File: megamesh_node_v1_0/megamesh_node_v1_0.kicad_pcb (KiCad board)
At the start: 2 copper layers, 85.5 x 60.5 mm, 4 parts, among them J1 Conn_Coaxial, U1 ESP32-S3-WROOM-1, U2 LoRa126XF30, U3 BQ25798

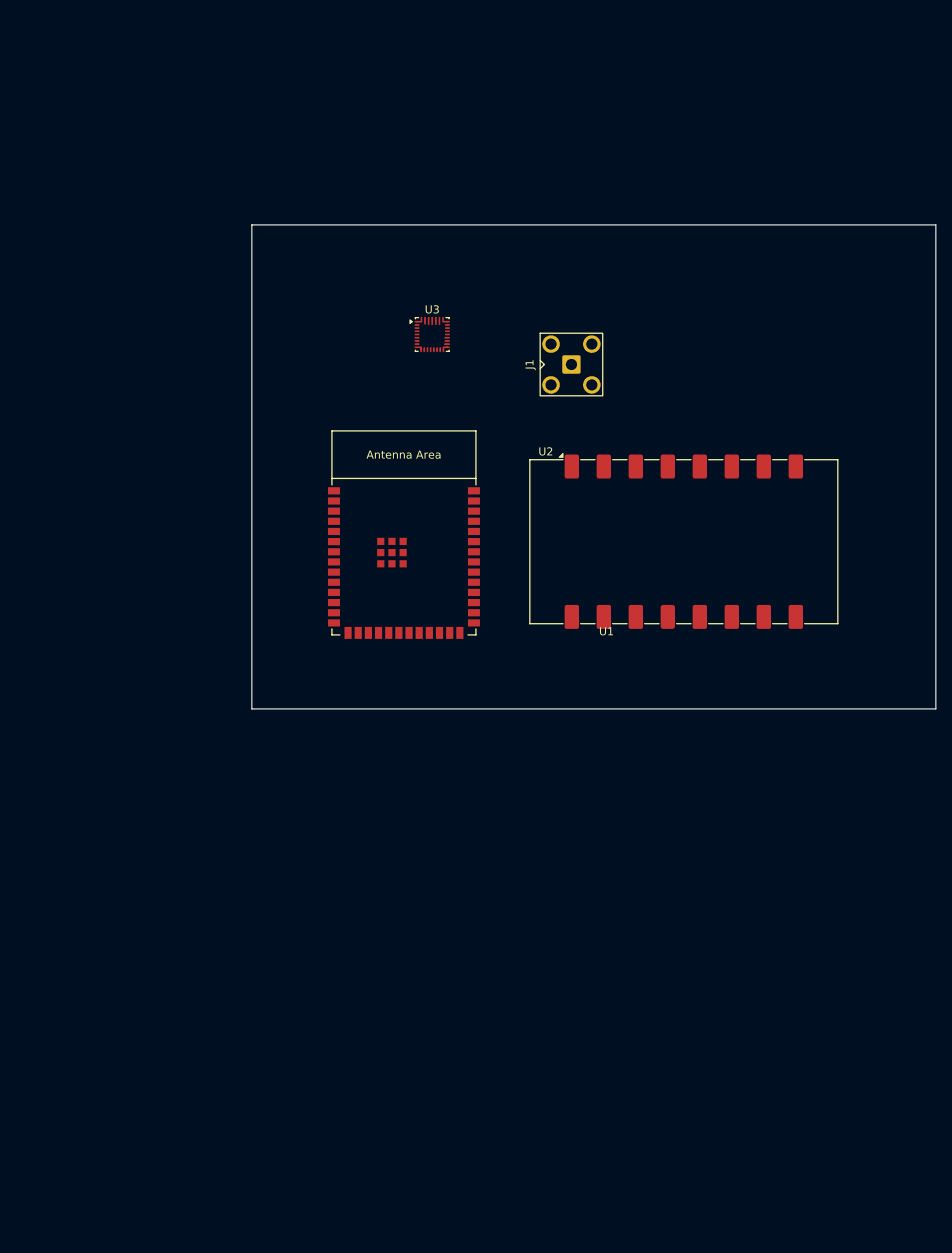
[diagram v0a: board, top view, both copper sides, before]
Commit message: Entwicklung Schaltplan und Platine
Es geht voran
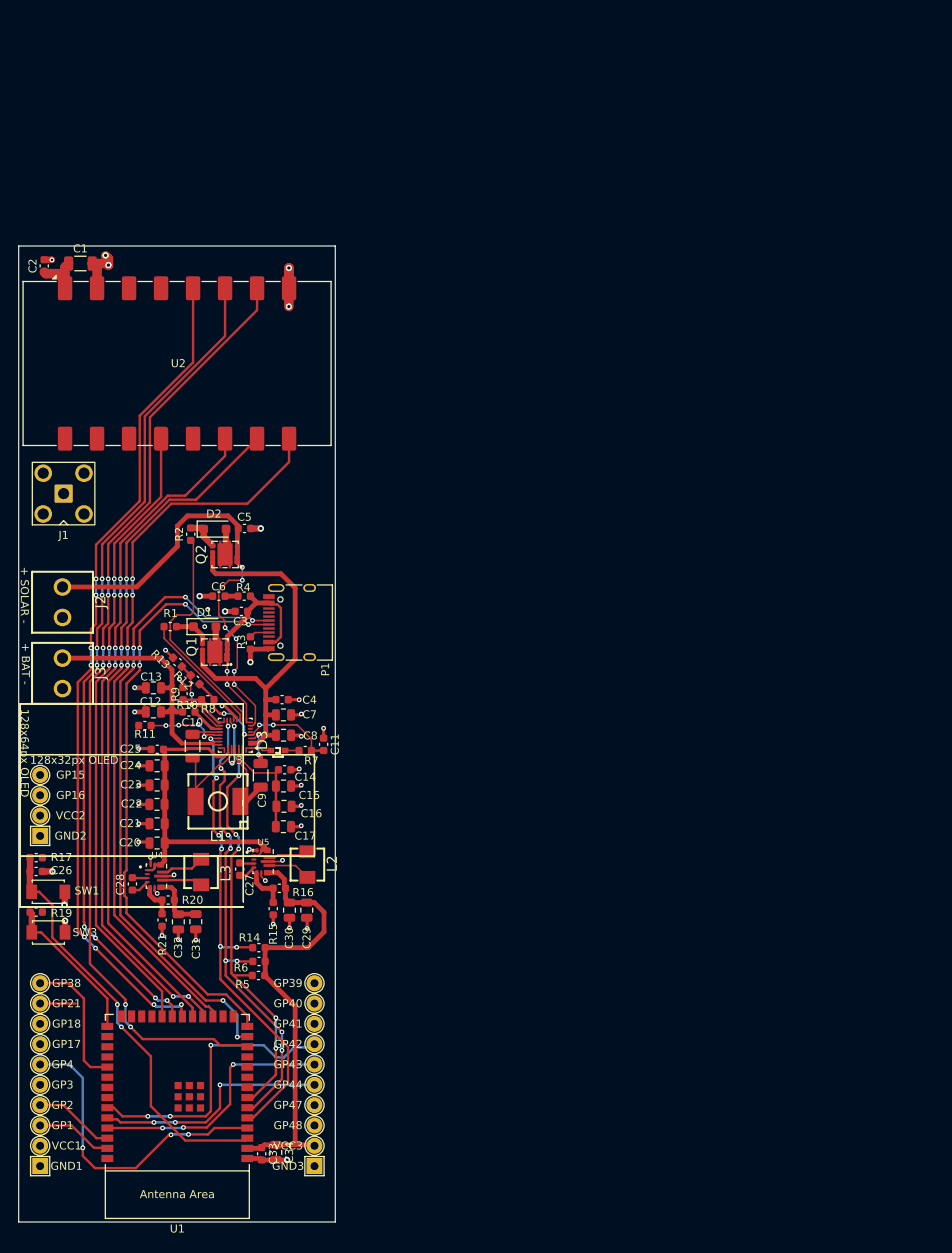
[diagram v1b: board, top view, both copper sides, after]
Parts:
- added C1: 47 uF, Capacitor_SMD:C_1206_3216Metric, F.Cu at (71.1, 71.3)
- added C10: 47 uF, Capacitor_SMD:C_1206_3216Metric, F.Cu at (85.1, 131.7)
- added C11: 47 nF, Capacitor_SMD:C_0603_1608Metric, F.Cu at (101.5, 131.4)
- added C12: 10 uF, Capacitor_SMD:C_0805_2012Metric, F.Cu at (80.2, 127.4)
- added C13: 10 uF, Capacitor_SMD:C_0805_2012Metric, F.Cu at (80.2, 124.4)
- added C14: 0.1 uF, Capacitor_SMD:C_0603_1608Metric, F.Cu at (96.6, 134.6)
- added C15: 10 uF, Capacitor_SMD:C_0805_2012Metric, F.Cu at (96.5, 136.6)
- added C16: 10 uF, Capacitor_SMD:C_0805_2012Metric, F.Cu at (96.5, 139.2)
- added C17: 10 uF, Capacitor_SMD:C_0805_2012Metric, F.Cu at (96.4, 141.7)
- added C2: 100 nF, Capacitor_SMD:C_0603_1608Metric, F.Cu at (66.5, 71.6)
- added C20: 10 uF, Capacitor_SMD:C_0805_2012Metric, F.Cu at (80.7, 143.8)
- added C21: 10 uF, Capacitor_SMD:C_0805_2012Metric, F.Cu at (80.7, 141.4)
- added C22: 10 uF, Capacitor_SMD:C_0805_2012Metric, F.Cu at (80.6, 138.9)
- added C23: 10 uF, Capacitor_SMD:C_0805_2012Metric, F.Cu at (80.7, 136.5)
- added C24: 10 uF, Capacitor_SMD:C_0805_2012Metric, F.Cu at (80.7, 134.1)
- added C25: 0.1 uF, Capacitor_SMD:C_0603_1608Metric, F.Cu at (80.7, 132.1)
- added C26: 100 nF, Capacitor_SMD:C_0603_1608Metric, F.Cu at (65.5, 147.3)
- added C27: 1 uF, Capacitor_SMD:C_0603_1608Metric, F.Cu at (91.0, 147.0)
- added C28: 1 uF, Capacitor_SMD:C_0603_1608Metric, F.Cu at (77.6, 148.9)
- added C29: 22 uF, Capacitor_SMD:C_0805_2012Metric, F.Cu at (99.4, 152.2)
- added C3: 0.1uF, Capacitor_SMD:C_0603_1608Metric, F.Cu at (91.2, 114.8)
- added C30: 22 uF, Capacitor_SMD:C_0805_2012Metric, F.Cu at (97.2, 152.2)
- added C31: 22 uF, Capacitor_SMD:C_0805_2012Metric, F.Cu at (85.5, 153.6)
- added C32: 22 uF, Capacitor_SMD:C_0805_2012Metric, F.Cu at (83.3, 153.6)
- added C33: 100 nF, Capacitor_SMD:C_0603_1608Metric, F.Cu at (93.7, 182.6)
- added C34: 10 uF, Capacitor_SMD:C_0805_2012Metric, F.Cu at (95.5, 182.4)
- added C4: 0.1 uF, Capacitor_SMD:C_0603_1608Metric, F.Cu at (96.3, 125.8)
- added C5: 0.1uF, Capacitor_SMD:C_0603_1608Metric, F.Cu at (91.6, 104.4)
- added C6: 2.2 uF, Capacitor_SMD:C_0603_1608Metric, F.Cu at (88.4, 112.9)
- added C7: 10 uF, Capacitor_SMD:C_0805_2012Metric, F.Cu at (96.5, 127.7)
- added C8: 10 uF, Capacitor_SMD:C_0805_2012Metric, F.Cu at (96.5, 130.3)
- added C9: 47 uF, Capacitor_SMD:C_1206_3216Metric, F.Cu at (93.6, 135.3)
- added D1: BZT52BC12, Diode_SMD:D_SOD-123F, F.Cu at (86.6, 116.7)
- added D2: BZT52BC12, Diode_SMD:D_SOD-123F, F.Cu at (87.9, 104.5)
- added D3: LED, myRF:LED-SMD_L1.7-W0.6-R-RD, F.Cu at (95.8, 132.2)
- added GND1: GND, TestPoint:TestPoint_THTPad_2.0x2.0mm_Drill1.0mm, F.Cu at (66.0, 184.2)
- added GND2: GND, TestPoint:TestPoint_THTPad_2.0x2.0mm_Drill1.0mm, F.Cu at (66.0, 142.9)
- added GND3: GND, TestPoint:TestPoint_THTPad_2.0x2.0mm_Drill1.0mm, F.Cu at (100.3, 184.2)
- added GP1: GPIO1, TestPoint:TestPoint_THTPad_D2.0mm_Drill1.0mm, F.Cu at (66.0, 179.1)
- added GP15: I2C SDA, TestPoint:TestPoint_THTPad_D2.0mm_Drill1.0mm, F.Cu at (66.0, 135.3)
- added GP16: I2C SCL, TestPoint:TestPoint_THTPad_D2.0mm_Drill1.0mm, F.Cu at (66.0, 137.8)
- added GP17: GPIO17, TestPoint:TestPoint_THTPad_D2.0mm_Drill1.0mm, F.Cu at (66.0, 168.9)
- added GP18: GPIO18, TestPoint:TestPoint_THTPad_D2.0mm_Drill1.0mm, F.Cu at (66.0, 166.4)
- added GP2: GPIO2, TestPoint:TestPoint_THTPad_D2.0mm_Drill1.0mm, F.Cu at (66.0, 176.5)
- added GP21: GPIO21, TestPoint:TestPoint_THTPad_D2.0mm_Drill1.0mm, F.Cu at (66.0, 163.8)
- added GP3: GPIO3, TestPoint:TestPoint_THTPad_D2.0mm_Drill1.0mm, F.Cu at (66.0, 174.0)
- added GP38: GPIO38, TestPoint:TestPoint_THTPad_D2.0mm_Drill1.0mm, F.Cu at (66.0, 161.3)
- added GP39: GPIO39, TestPoint:TestPoint_THTPad_D2.0mm_Drill1.0mm, F.Cu at (100.3, 161.3)
- added GP4: GPIO4, TestPoint:TestPoint_THTPad_D2.0mm_Drill1.0mm, F.Cu at (66.0, 171.4)
- added GP40: GPIO40, TestPoint:TestPoint_THTPad_D2.0mm_Drill1.0mm, F.Cu at (100.3, 163.8)
- added GP41: GPIO41, TestPoint:TestPoint_THTPad_D2.0mm_Drill1.0mm, F.Cu at (100.3, 166.4)
- added GP42: GPIO42, TestPoint:TestPoint_THTPad_D2.0mm_Drill1.0mm, F.Cu at (100.3, 168.9)
- added GP43: TX0, TestPoint:TestPoint_THTPad_D2.0mm_Drill1.0mm, F.Cu at (100.3, 171.4)
- added GP44: RX0, TestPoint:TestPoint_THTPad_D2.0mm_Drill1.0mm, F.Cu at (100.3, 174.0)
- added GP47: GPIO47, TestPoint:TestPoint_THTPad_D2.0mm_Drill1.0mm, F.Cu at (100.3, 176.5)
- added GP48: GPIO48, TestPoint:TestPoint_THTPad_D2.0mm_Drill1.0mm, F.Cu at (100.3, 179.1)
- added J2: Screw_Terminal_01x02, myRF:CONN-TH_2P-P3.81_KF124-3.81-2P, F.Cu at (68.8, 113.7)
- added J3: Screw_Terminal_01x02, myRF:CONN-TH_2P-P3.81_KF124-3.81-2P, F.Cu at (68.8, 122.6)
- added L1: 1.0 uH, myRF:IND-SMD_L7.1-W6.5-P5.60, F.Cu at (88.3, 138.6)
- added L2: 1.5 uH, myRF:IND-SMD_L4.2-W4.0_SPM4030T, F.Cu at (99.4, 146.5)
- added L3: 1.5 uH, myRF:IND-SMD_L4.2-W4.0_SPM4030T, F.Cu at (86.2, 147.4)
- added P1: USB_C_Plug_USB2.0, Connector_USB:USB_C_Receptacle_HRO_TYPE-C-31-M-12, F.Cu at (98.7, 116.2)
- added Q1: CSD87312Q3E, myRF:SON 3.3x3.3mm, F.Cu at (87.9, 119.9)
- added Q2: CSD87312Q3E, myRF:SON 3.3x3.3mm, F.Cu at (89.2, 107.7)
- added R1: 294 Ohm, Capacitor_SMD:C_0603_1608Metric, F.Cu at (82.3, 116.7)
- added R10: 100 Ohm, Capacitor_SMD:C_0603_1608Metric, F.Cu at (84.6, 127.4)
- added R11: 6.04 kOhm, Capacitor_SMD:C_0603_1608Metric, F.Cu at (79.1, 129.1)
- added R12: 127 kOhm, Capacitor_SMD:C_0603_1608Metric, F.Cu at (85.4, 123.4)
- added R13: 127 kOhm, Capacitor_SMD:C_0603_1608Metric, F.Cu at (83.2, 121.2)
- added R14: 4.7 kOhm, Capacitor_SMD:C_0603_1608Metric, F.Cu at (93.4, 156.8)
- added R15: 200 kOhm, Capacitor_SMD:C_0603_1608Metric, F.Cu at (95.2, 152.0)
- added R16: 624 kOhm, Capacitor_SMD:C_0603_1608Metric, F.Cu at (95.9, 149.4)
- added R17: 10 kOhm, Capacitor_SMD:C_0603_1608Metric, F.Cu at (65.5, 145.6)
- added R19: 10 kOhm, Capacitor_SMD:C_0603_1608Metric, F.Cu at (65.5, 152.4)
- added R2: 294 Ohm, Capacitor_SMD:C_0603_1608Metric, F.Cu at (84.9, 105.2)
- added R20: 649 kOhm, Capacitor_SMD:C_0603_1608Metric, F.Cu at (82.0, 150.9)
- added R21: 100 kOhm, Capacitor_SMD:C_0603_1608Metric, F.Cu at (81.3, 153.4)
- added R3: 5.1 kOhm, Capacitor_SMD:C_0603_1608Metric, F.Cu at (92.3, 118.8)
- added R4: 2 Ohm, Capacitor_SMD:C_0603_1608Metric, F.Cu at (91.5, 112.9)
- added R5: 4.7 kOhm, Capacitor_SMD:C_0603_1608Metric, F.Cu at (93.3, 160.3)
- added R6: 4.7 kOhm, Capacitor_SMD:C_0603_1608Metric, F.Cu at (93.4, 158.6)
- added R7: 2.2 kOhm, Capacitor_SMD:C_0603_1608Metric, F.Cu at (99.2, 132.2)
- added R8: 10 kOhm, Capacitor_SMD:C_0603_1608Metric, F.Cu at (87.0, 125.9)
- added R9: 10 kOhm, Capacitor_SMD:C_0603_1608Metric, F.Cu at (83.9, 125.1)
- added SW1: SW_Push, myRF:SW_TS-1088-AR02016, F.Cu at (67.1, 149.9)
- added SW3: SW_Push, myRF:SW_TS-1088-AR02016, F.Cu at (67.1, 154.9)
- added U4: TPS63070RNMR, TPS63070RNMR:VREG_TPS63070RNMR, F.Cu at (80.6, 147.9)
- added U5: TPS63070RNMR, TPS63070RNMR:VREG_TPS63070RNMR, F.Cu at (93.9, 146.1)
- added VCC1: 3v3, TestPoint:TestPoint_THTPad_D2.0mm_Drill1.0mm, F.Cu at (66.0, 181.6)
- added VCC2: 3v3, TestPoint:TestPoint_THTPad_D2.0mm_Drill1.0mm, F.Cu at (66.0, 140.3)
- added VCC3: 3v3, TestPoint:TestPoint_THTPad_D2.0mm_Drill1.0mm, F.Cu at (100.3, 181.6)
- moved U1 72.7 mm to (83.2, 174.9), turned to 180 degrees
- moved U2 67.1 mm to (83.2, 83.8)
- moved J1 65.5 mm to (69.0, 100.1), turned to 90 degrees
- moved U3 55.8 mm to (90.4, 130.3), turned to 180 degrees
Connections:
- net Net-(U3-VBUS-Pad2) renamed D2
- U1 pad 10: unconnected-(U1-GPIO17/U1TXD/ADC2_CH6-Pad10) -> Net-(U1-GPIO17/U1TXD/ADC2_CH6)
- U1 pad 11: unconnected-(U1-GPIO18/U1RXD/ADC2_CH7/CLK_OUT3-Pad11) -> Net-(U1-GPIO18/U1RXD/ADC2_CH7/CLK_OUT3)
- U1 pad 12: unconnected-(U1-GPIO8/TOUCH8/ADC1_CH7/SUBSPICS1-Pad12) -> NSS
- U1 pad 13: unconnected-(U1-GPIO19/U1RTS/ADC2_CH8/CLK_OUT2/USB_D--Pad13) -> D-
- U1 pad 14: unconnected-(U1-GPIO20/U1CTS/ADC2_CH9/CLK_OUT1/USB_D+-Pad14) -> D+
- U1 pad 15: unconnected-(U1-GPIO3/TOUCH3/ADC1_CH2-Pad15) -> Net-(U1-GPIO3/TOUCH3/ADC1_CH2)
- U1 pad 17: unconnected-(U1-GPIO9/TOUCH9/ADC1_CH8/FSPIHD/SUBSPIHD-Pad17) -> SCK
- U1 pad 18: unconnected-(U1-GPIO10/TOUCH10/ADC1_CH9/FSPICS0/FSPIIO4/SUBSPICS0-Pad18) -> MOSI
- U1 pad 19: unconnected-(U1-GPIO11/TOUCH11/ADC2_CH0/FSPID/FSPIIO5/SUBSPID-Pad19) -> MISO
- U1 pad 2: unconnected-(U1-3V3-Pad2) -> +3V3
- U1 pad 20: unconnected-(U1-GPIO12/TOUCH12/ADC2_CH1/FSPICLK/FSPIIO6/SUBSPICLK-Pad20) -> NRESET
- U1 pad 21: unconnected-(U1-GPIO13/TOUCH13/ADC2_CH2/FSPIQ/FSPIIO7/SUBSPIQ-Pad21) -> BUSY
- U1 pad 22: unconnected-(U1-GPIO14/TOUCH14/ADC2_CH3/FSPIWP/FSPIDQS/SUBSPIWP-Pad22) -> DIO0
- U1 pad 23: unconnected-(U1-GPIO21-Pad23) -> Net-(U1-GPIO21)
- U1 pad 24: unconnected-(U1-GPIO47/SPICLK_P/SUBSPICLK_P_DIFF-Pad24) -> Net-(U1-GPIO47/SPICLK_P/SUBSPICLK_P_DIFF)
- U1 pad 25: unconnected-(U1-GPIO48/SPICLK_N/SUBSPICLK_N_DIFF-Pad25) -> Net-(U1-GPIO48/SPICLK_N/SUBSPICLK_N_DIFF)
- U1 pad 27: unconnected-(U1-GPIO0/BOOT-Pad27) -> BOOT_SW
- U1 pad 3: unconnected-(U1-EN-Pad3) -> EN_SW
- U1 pad 31: unconnected-(U1-GPIO38/FSPIWP/SUBSPIWP-Pad31) -> Net-(U1-GPIO38/FSPIWP/SUBSPIWP)
- U1 pad 32: unconnected-(U1-MTCK/GPIO39/CLK_OUT3/SUBSPICS1-Pad32) -> Net-(U1-MTCK/GPIO39/CLK_OUT3/SUBSPICS1)
- U1 pad 33: unconnected-(U1-MTDO/GPIO40/CLK_OUT2-Pad33) -> Net-(U1-MTDO/GPIO40/CLK_OUT2)
- U1 pad 34: unconnected-(U1-MTDI/GPIO41/CLK_OUT1-Pad34) -> Net-(U1-MTDI/GPIO41/CLK_OUT1)
- U1 pad 35: unconnected-(U1-MTMS/GPIO42-Pad35) -> Net-(U1-MTMS/GPIO42)
- U1 pad 36: unconnected-(U1-U0RXD/GPIO44/CLK_OUT2-Pad36) -> Net-(U1-U0RXD/GPIO44/CLK_OUT2)
- U1 pad 37: unconnected-(U1-U0TXD/GPIO43/CLK_OUT1-Pad37) -> Net-(U1-U0TXD/GPIO43/CLK_OUT1)
- U1 pad 38: unconnected-(U1-GPIO2/TOUCH2/ADC1_CH1-Pad38) -> Net-(U1-GPIO2/TOUCH2/ADC1_CH1)
- U1 pad 39: unconnected-(U1-GPIO1/TOUCH1/ADC1_CH0-Pad39) -> Net-(U1-GPIO1/TOUCH1/ADC1_CH0)
- U1 pad 4: unconnected-(U1-GPIO4/TOUCH4/ADC1_CH3-Pad4) -> Net-(U1-GPIO4/TOUCH4/ADC1_CH3)
- U1 pad 5: unconnected-(U1-GPIO5/TOUCH5/ADC1_CH4-Pad5) -> !INT
- U1 pad 6: unconnected-(U1-GPIO6/TOUCH6/ADC1_CH5-Pad6) -> SDA
- U1 pad 7: unconnected-(U1-GPIO7/TOUCH7/ADC1_CH6-Pad7) -> SCL
- U1 pad 8: unconnected-(U1-GPIO15/U0RTS/ADC2_CH4/XTAL_32K_P-Pad8) -> Net-(U1-GPIO15/U0RTS/ADC2_CH4/XTAL_32K_P)
- U1 pad 9: unconnected-(U1-GPIO16/U0CTS/ADC2_CH5/XTAL_32K_N-Pad9) -> Net-(U1-GPIO16/U0CTS/ADC2_CH5/XTAL_32K_N)
- U2 pad 1: +5V -> +6V
- U2 pad 10: unconnected-(U2-MISO-Pad10) -> MISO
- U2 pad 11: unconnected-(U2-MOSI-Pad11) -> MOSI
- U2 pad 13: unconnected-(U2-DIO1-Pad13) -> DIO0
- U2 pad 5: unconnected-(U2-NRESET-Pad5) -> NRESET
- U2 pad 6: unconnected-(U2-BUSY-Pad6) -> BUSY
- U2 pad 7: unconnected-(U2-NSS-Pad7) -> NSS
- U2 pad 8: unconnected-(U2-GND-Pad8) -> GND
- U2 pad 9: unconnected-(U2-SCK-Pad9) -> SCK
- U3 pad 1: unconnected-(U3-STAT-Pad1) -> Net-(D3-K)
- U3 pad 10: unconnected-(U3-ACDRV2-Pad10) -> Gate_ACDRV2
- U3 pad 11: unconnected-(U3-ACDRV1-Pad11) -> Gate_ACDRV1
- U3 pad 12: unconnected-(U3-~{QON}-Pad12) -> GND
- U3 pad 13: unconnected-(U3-~{CE}-Pad13) -> GND
- U3 pad 14: unconnected-(U3-SCL-Pad14) -> SCL
- U3 pad 15: unconnected-(U3-SDA-Pad15) -> SDA
- U3 pad 16: unconnected-(U3-TS-Pad16) -> Net-(U3-TS)
- U3 pad 17: unconnected-(U3-ILIM_HIZ-Pad17) -> Net-(U3-ILIM_HIZ)
- U3 pad 18: unconnected-(U3-BATP-Pad18) -> Net-(U3-BATP)
- U3 pad 19: unconnected-(U3-BTST2-Pad19) -> Net-(U3-BTST2)
- U3 pad 20: unconnected-(U3-PROG-Pad20) -> Net-(U3-PROG)
- U3 pad 21: unconnected-(U3-~{INT}-Pad21) -> !INT
- U3 pad 25: unconnected-(U3-SYS-Pad25) -> SYS
- U3 pad 26: unconnected-(U3-SW2-Pad26) -> Net-(U3-SW2)
- U3 pad 28: unconnected-(U3-SW1-Pad28) -> Net-(U3-SW1)
- U3 pad 29: unconnected-(U3-PMID-Pad29) -> Net-(U3-PMID)
- U3 pad 4: unconnected-(U3-BTST1-Pad4) -> Net-(U3-BTST1)
- U3 pad 5: unconnected-(U3-REGN-Pad5) -> REGN
- U3 pad 8: unconnected-(U3-VAC2-Pad8) -> D1_VAC2
- U3 pad 9: unconnected-(U3-VAC1-Pad9) -> D1_VAC1
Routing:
- net NSS: track 0.00 -> 118.7 mm, vias 0 -> 6
- net NRESET: track 0.00 -> 105.2 mm, vias 0 -> 8
- net BUSY: track 0.00 -> 103.5 mm, vias 0 -> 8
- net SCK: track 0.00 -> 92.2 mm, vias 0 -> 4
- net MOSI: track 0.00 -> 86.3 mm, vias 0 -> 6
- net MISO: track 0.00 -> 86.2 mm, vias 0 -> 4
- net GND: track 0.00 -> 84.4 mm, vias 0 -> 47
- net D-: track 0.00 -> 80.1 mm, vias 0 -> 6
- net DIO0: track 0.00 -> 79.0 mm, vias 0 -> 4
- net D+: track 0.00 -> 76.5 mm, vias 0 -> 4
- net !INT: track 0.00 -> 59.8 mm, vias 0 -> 6
- net SDA: track 0.00 -> 58.9 mm, vias 0 -> 8
- net D1_VAC2: track 0.00 -> 57.4 mm, vias 0 -> 6
- net +3V3: track 0.00 -> 56.0 mm
- net SCL: track 0.00 -> 55.8 mm, vias 0 -> 6
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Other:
- board size 85.5 x 60.5 mm -> 39.6 x 122 mm
- board text added: "+ BAT -"
- board text added: "+ SOLAR -"
- board text added: "128x32px OLED"
- board text added: "128x64px OLED"

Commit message: Fertigstellung
I guess
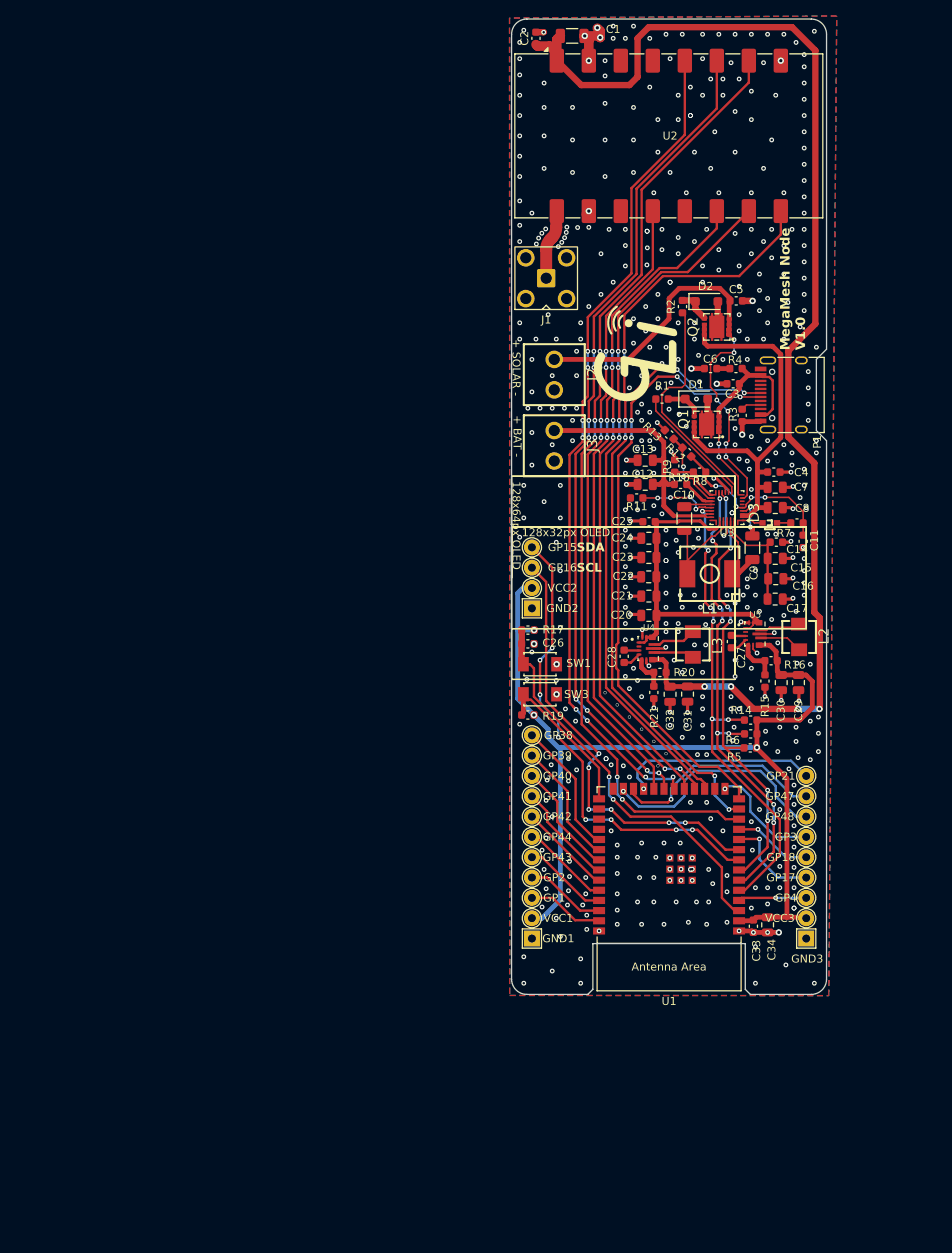
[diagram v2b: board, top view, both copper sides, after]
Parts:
- added G***: LOGO, LOGO, F.Cu at (140.5, 82.5)
- moved GP3 100.6 mm to (161.8, 143.0)
- moved GP21 99.9 mm to (161.8, 135.4)
- moved GP17 98.0 mm to (161.8, 148.1)
- moved GP18 98.0 mm to (161.8, 145.5)
- moved GP4 98.0 mm to (161.8, 150.6)
- moved GP47 72.6 mm to (161.8, 137.9)
- moved GP48 72.6 mm to (161.8, 140.5)
- moved GP38 68.8 mm to (127.5, 130.3)
- moved SW3 68.3 mm to (128.5, 125.2)
- moved C15 67.7 mm to (157.9, 108.2)
- moved C3 67.7 mm to (152.7, 86.4)
- moved R5 67.7 mm to (154.8, 131.9)
- moved U5 67.7 mm to (155.4, 117.6)
- moved C28 67.7 mm to (139.0, 120.4)
- moved C30 67.7 mm to (158.7, 123.7)
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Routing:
- net +6V: track 14.5 -> 158.2 mm, vias 0 -> 4
- net +3V3: track 56.0 -> 129.5 mm, vias 0 -> 3
- net Net-(U1-GPIO15/U0RTS/ADC2_CH4/XTAL_32K_P): track 0.00 -> 59.1 mm, vias 0 -> 8
- net Net-(U1-GPIO16/U0CTS/ADC2_CH5/XTAL_32K_N): track 0.00 -> 55.1 mm, vias 0 -> 6
- net Net-(U1-GPIO4/TOUCH4/ADC1_CH3): track 39.1 -> 8.53 mm, vias 3 -> 1
- net Net-(U1-GPIO48/SPICLK_N/SUBSPICLK_N_DIFF): track 0.00 -> 30.1 mm, vias 0 -> 1
- net Net-(U1-GPIO47/SPICLK_P/SUBSPICLK_P_DIFF): track 0.00 -> 27.0 mm, vias 0 -> 1
- net Net-(U1-MTMS/GPIO42): track 36.3 -> 11.7 mm, vias 3 -> 0
- net Net-(U1-U0TXD/GPIO43/CLK_OUT1): track 32.0 -> 10.6 mm, vias 3 -> 0
- net Net-(U1-GPIO21): track 4.44 -> 25.0 mm, vias 0 -> 1
- net Net-(U1-U0RXD/GPIO44/CLK_OUT2): track 29.8 -> 11.2 mm, vias 3 -> 0
- net Net-(U1-MTCK/GPIO39/CLK_OUT3/SUBSPICS1): track 0.00 -> 15.5 mm
- net Net-(U1-MTDO/GPIO40/CLK_OUT2): track 0.00 -> 14.2 mm
- net Net-(U1-GPIO3/TOUCH3/ADC1_CH2): track 0.00 -> 14.0 mm, vias 0 -> 1
- net Net-(U1-MTDI/GPIO41/CLK_OUT1): track 0.00 -> 13.0 mm
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- added copper zone on B.Cu, net GND
- added copper zone on F.Cu, net GND
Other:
- board size 39.6 x 122 mm -> 39.4 x 121.9 mm
- board text added: "MegaMesh Node V1.0"
- board text added: "SCL"
- board text added: "SDA"
